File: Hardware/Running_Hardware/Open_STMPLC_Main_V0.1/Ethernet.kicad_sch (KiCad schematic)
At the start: 16 parts, among them J11 HY951180A, U7 LAN8720A

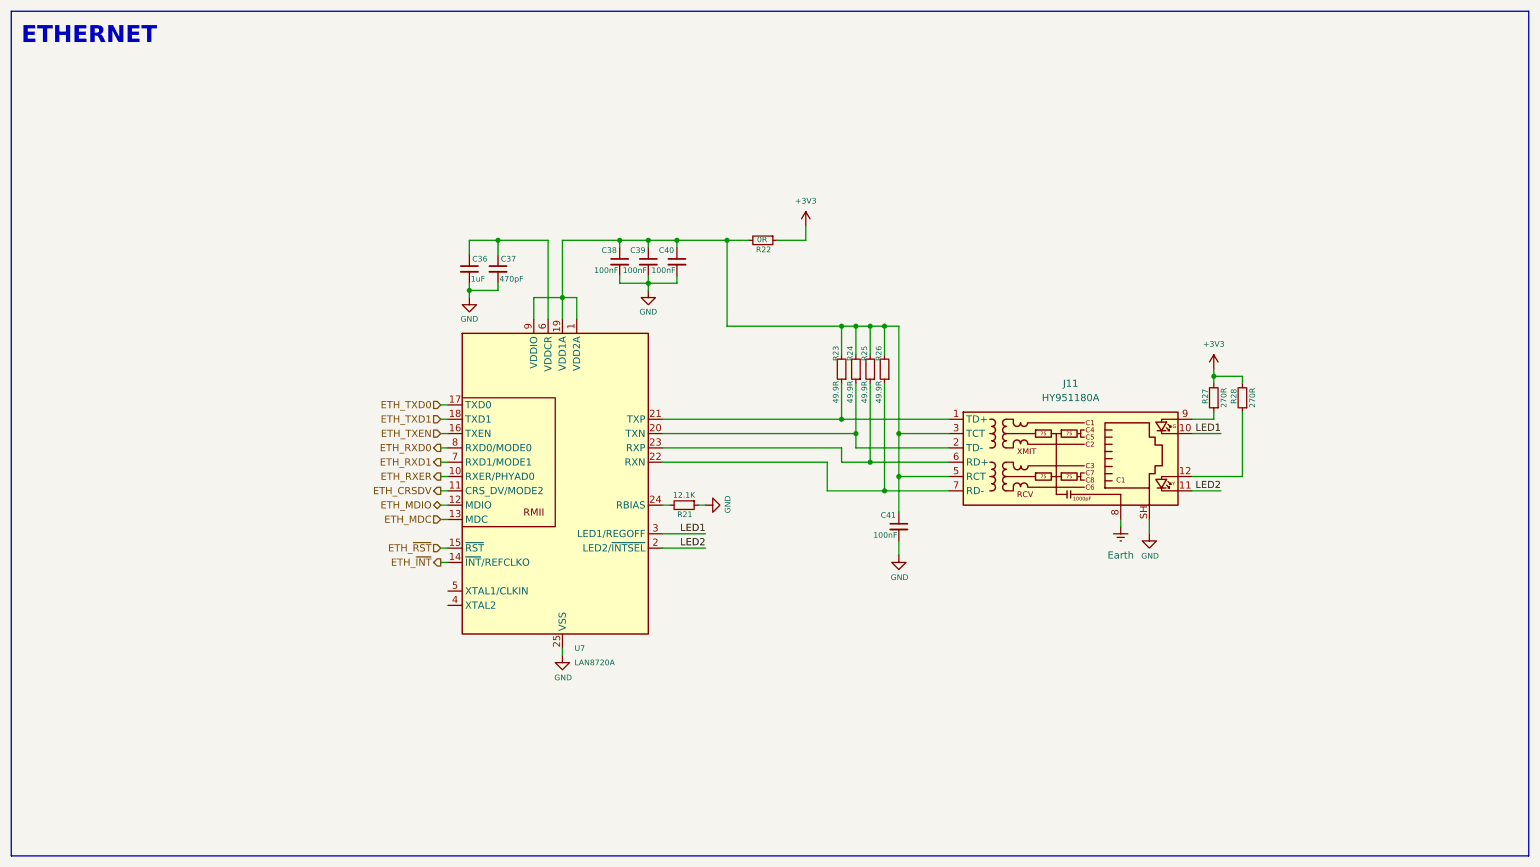
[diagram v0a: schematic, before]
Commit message: Main PCB changes
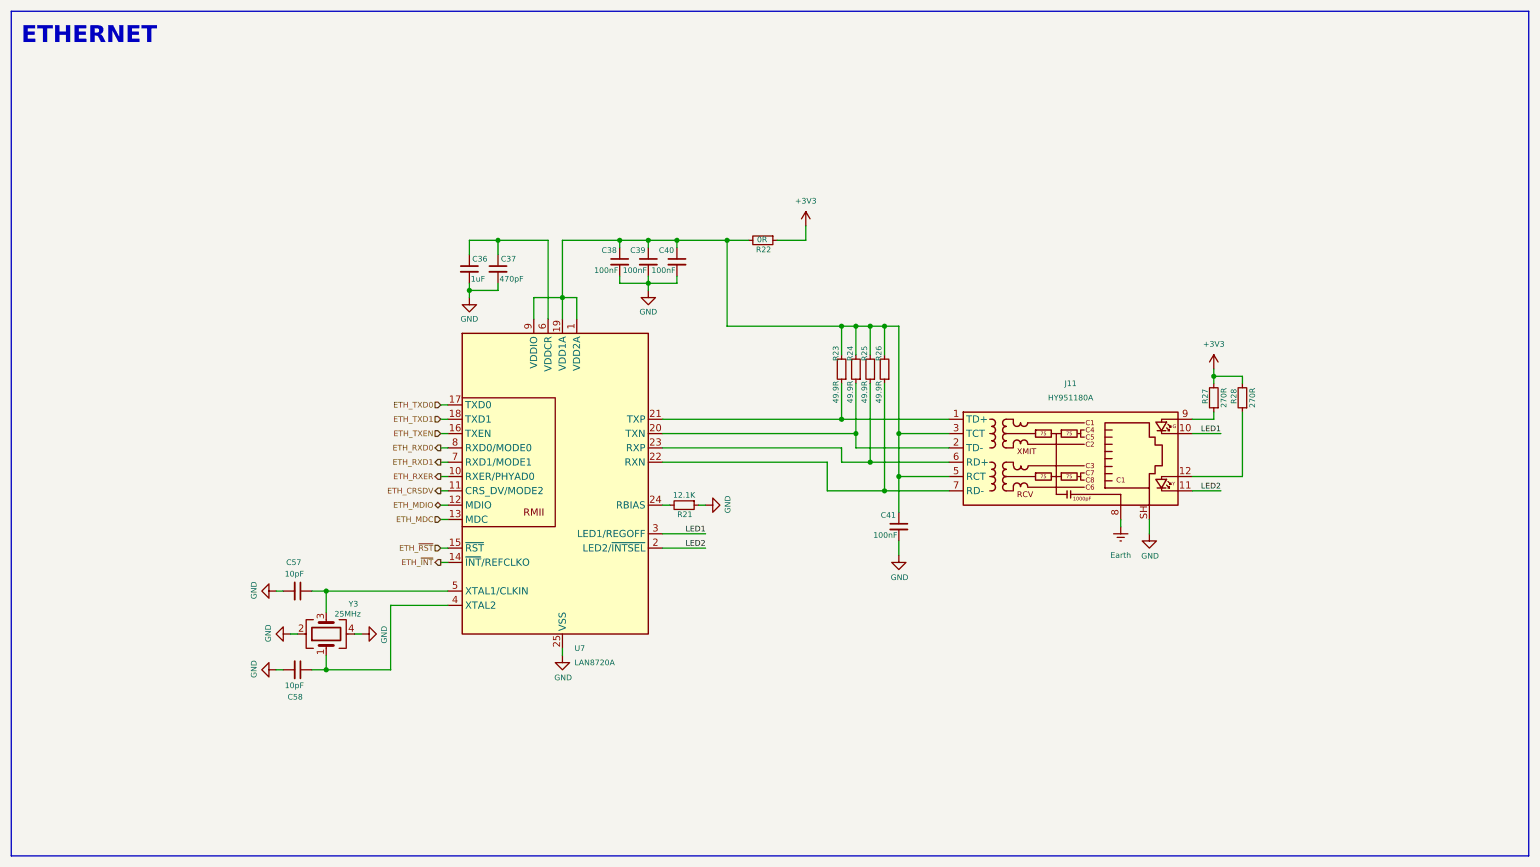
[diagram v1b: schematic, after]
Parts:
- added C57, C58: 10pF, Capacitor_SMD:C_0603_1608Metric_Pad1.08x0.95mm_HandSolder, symbol Device:C_Small
- added Y3: 25MHz, Crystal:Crystal_SMD_5032-4Pin_5.0x3.2mm, symbol Device:Crystal_GND24
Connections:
- net GND: now also C57.2, C58.2, Y3.2, Y3.4
- net at U7.4 (XTAL2): now also C58.1, Y3.1
- net at U7.5 (XTAL1/CLKIN): now also C57.1, Y3.3
